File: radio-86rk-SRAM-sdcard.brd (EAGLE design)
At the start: 49.2 x 49.5 mm, 15 parts, among them IC1 LM1117 3.3V, U1 ATMEGA328P, U2 HEF4050B

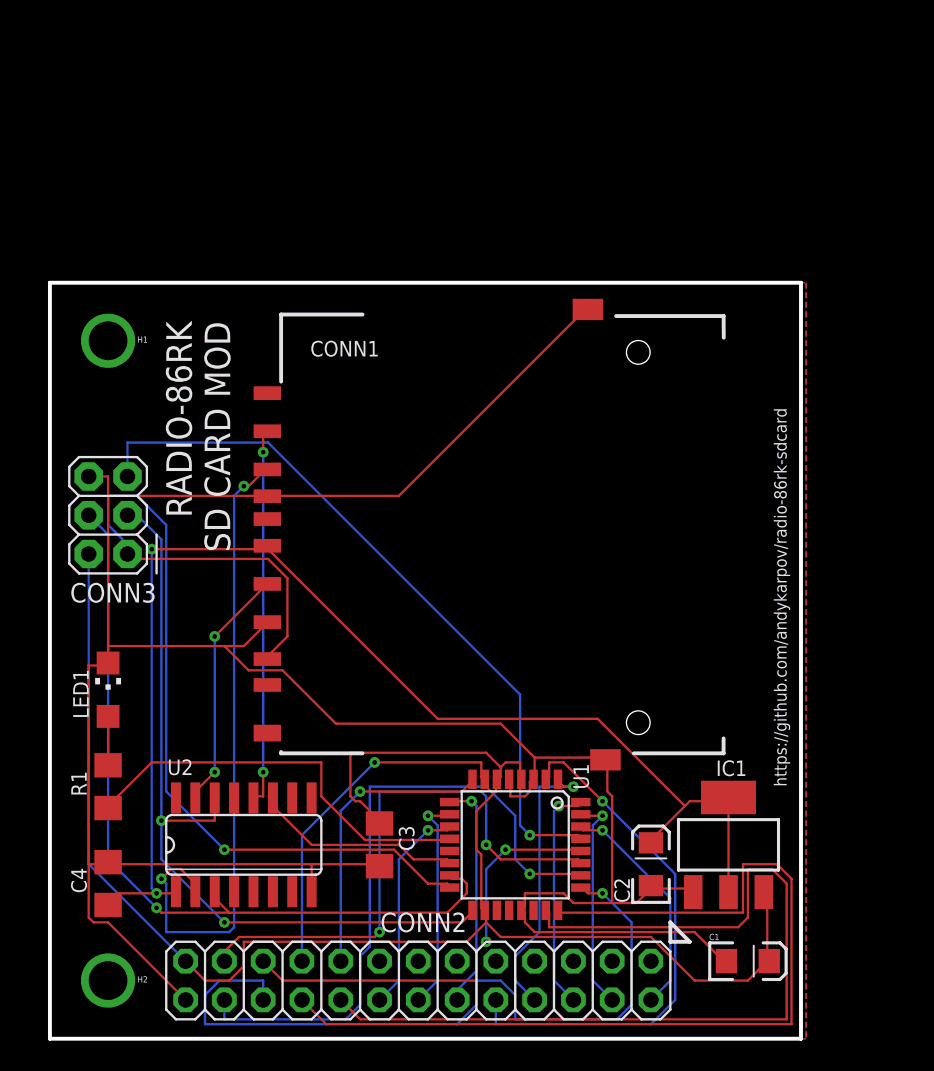
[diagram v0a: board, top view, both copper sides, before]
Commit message: Recovered v2.0 of the PCB
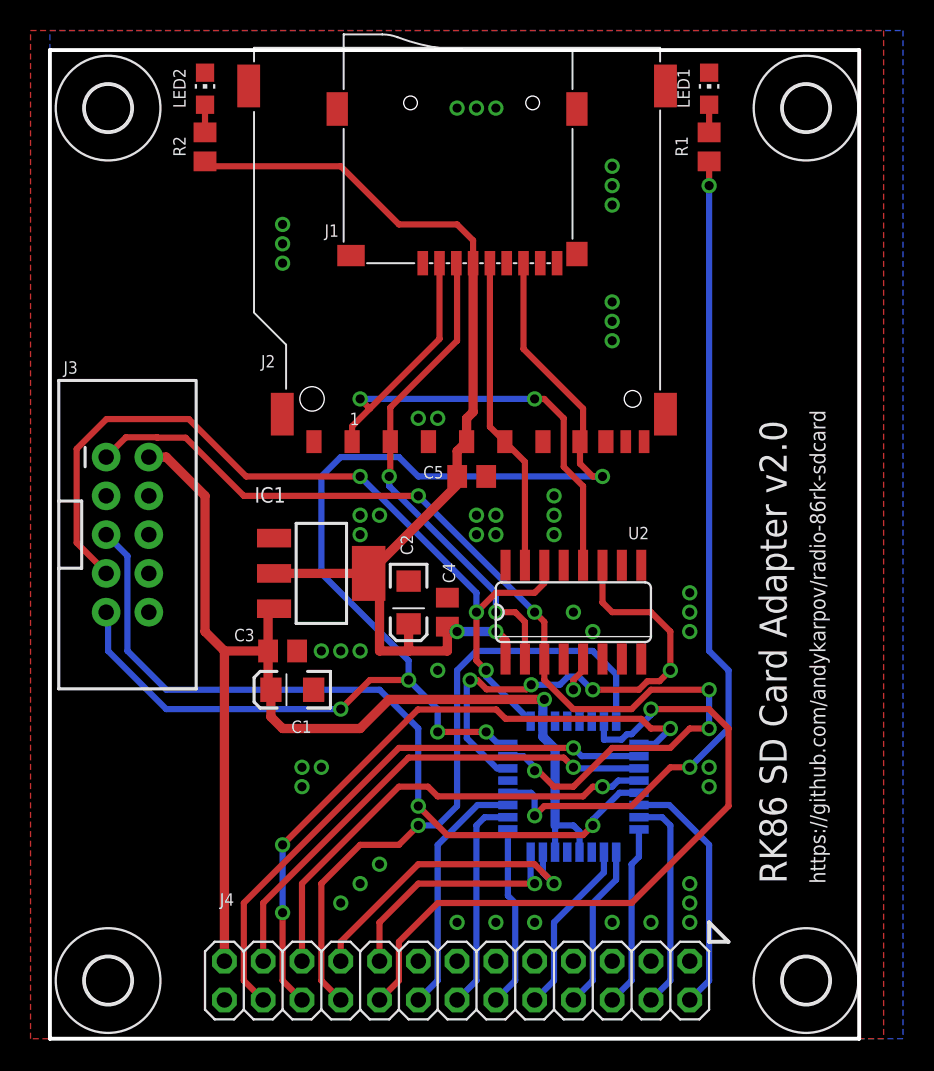
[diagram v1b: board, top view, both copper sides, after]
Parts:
- removed CONN1: SD CARD, SparkFun-Connectors:SDCARD_4UCONN
- removed CONN2: BUS, 2x13header:2X13
- removed CONN3: ISP, SparkFun-Connectors:2X03
- removed FRAME1: FRAME-LETTER, SparkFun-Aesthetics:CREATIVE_COMMONS
- removed H1, H2: SEW_HOLE, LilyPad-Wearables:SIMPLE_HOLE
- added C5: 100n, rcl:C0805
- added H5, H6, H7, H8: MOUNT-HOLE3.0, holes:3,0
- added J1: MICROSD, OPL_Connector:MICRO-SD9+4P-SMD-16.1X14.5X1.85MM
- added J2: SD, Wurth_Elektronik_Electromechanic_Input-Output_Connectors_rev18b:693063010911
- added J3: AVR ISP, SparkFun-Connectors:2X5-SHROUDED_LOCK
- added J4: BUS, 2x13header:2X13
- added LED2: PWR, led:CHIP-LED0805
- added R2: 470R, rcl:R0805
- C3, C4: device SparkFun-Capacitors:1206 -> rcl:C0805
- LED1: value 1206 -> BUSY; device adafruit:CHIPLED_1206 -> led:CHIP-LED0805
- R1: device SparkFun-Passives:1206 -> rcl:R0805
- U1: value ATMEGA328P -> ATMEGA8
- moved R1 57.5 mm to (43.2, 58.4)
- moved LED1 55.7 mm to (43.2, 62.2)
- moved C1 34.7 mm to (15.9, 22.9), turned to 180 degrees
- moved IC1 32.1 mm to (17.8, 30.5), turned to 270 degrees
- moved C4 28.5 mm to (26.0, 27.9)
- moved U2 26.4 mm to (34.3, 27.9)
- moved C2 23.4 mm to (23.5, 28.6), turned to 270 degrees
- moved C3 14.2 mm to (15.2, 25.4), turned to 0 degrees
- moved U1 5.39 mm to (34.3, 16.5), flipped to the bottom, turned to 90 degrees
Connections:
- new net N$2: LED2.A, R2.1
- net 3V3: now also C5.1, J1.4, J2.4, R2.2; no longer CONN1.4
- net A0: now also J4.18; no longer CONN2.18
- net A1: now also J4.20; no longer CONN2.20
- net A10: now also J4.5; no longer CONN2.5
- net A11: now also J4.7; no longer CONN2.7
- net A12: now also J4.9; no longer CONN2.9
- net A13: now also J4.11; no longer CONN2.11
- net A14: now also J4.13; no longer CONN2.13
- net A15: now also J4.15; no longer CONN2.15
- net A2: now also J4.22; no longer CONN2.22
- net A3: now also J4.24; no longer CONN2.24
- net A4: now also J4.23; no longer CONN2.23
- net A5: now also J4.21; no longer CONN2.21
- net A6: now also J4.19; no longer CONN2.19
- net A7: now also J4.17; no longer CONN2.17
- net A8: now also J4.1; no longer CONN2.1
- net A9: now also J4.3; no longer CONN2.3
- net CLK: now also J3.7; no longer CONN3.3
- net D0: now also J4.2; no longer CONN2.2
- net D1: now also J4.4; no longer CONN2.4
- net D2: now also J4.6; no longer CONN2.6
- net D3: now also J4.8; no longer CONN2.8
- net D4: now also J4.10; no longer CONN2.10
- net D5: now also J4.12; no longer CONN2.12
- net D6: now also J4.14; no longer CONN2.14
- net D7: now also J4.16; no longer CONN2.16
- net GND: now also C5.2, J1.6, J1.G1, J1.G2, J1.G3, J1.G4, J2.3, J2.6, J2.Z1, J2.Z2, J2.Z3, J2.Z4, J3.10, J3.4, J3.6, J3.8, J4.26, LED2.C, U2.5, U2.7, U2.9; no longer CONN1.3, CONN1.6, CONN1.SH@1, CONN1.SH@2, CONN2.26, CONN3.6
- net MISO: now also J1.7, J2.7, J3.9; no longer CONN1.7, CONN3.1
- net MOSI: now also J3.1; no longer CONN3.4
- net RESET: now also J3.5; no longer CONN3.5
- net SD_CLK: now also J1.5, J2.5; no longer CONN1.5
- net SD_MOSI: now also J1.3, J2.2; no longer CONN1.2
- net SD_SDSEL: now also J1.2, J2.1; no longer CONN1.1
- net VCC: now also J3.2, J4.25; no longer CONN2.25, CONN3.2
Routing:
- net GND: track 179.6 -> 2.27 mm, vias 0 -> 50
- net LED: track 27.1 -> 55.9 mm, vias 0 -> 3
- net VCC: track 106.8 -> 78.4 mm, vias 0 -> 1
- net D4: track 34.7 -> 11.6 mm, vias 1 -> 0
- net MISO: track 64.6 -> 85.6 mm, vias 1 -> 5
- net SDSEL: track 13.7 -> 32.3 mm, vias 0 -> 4
- net A1: track 61.2 -> 42.7 mm, vias 0 -> 1
- net MOSI: track 52.3 -> 68.4 mm, vias 1 -> 5
- net SD_SDSEL: track 24.8 -> 39.0 mm
- net A0: track 59.2 -> 45.6 mm, vias 0 -> 1
- net 3V3: track 82.3 -> 69.4 mm
- net SD_MOSI: track 42.7 -> 32.2 mm
- net D3: track 18.6 -> 10.8 mm, vias 1 -> 0
- net A2: track 49.5 -> 42.7 mm, vias 1 -> 3
- net A3: track 43.0 -> 37.2 mm
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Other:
- board size 49.2 x 49.5 mm -> 53 x 64.8 mm
- board text added: "RK86 SD Card Adapter v2.0"
- board text added: "Ukraine 2019"
- board text removed: "RADIO-86RK SD CARD MOD"
